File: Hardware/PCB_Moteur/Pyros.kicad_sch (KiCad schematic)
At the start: 33 parts, among them J17 Screw_Terminal_01x04, Q1 SI5442DU-T1-GE3, Q2 SI5442DU-T1-GE3, Q3 MMBT3904, Q4 SI7617DN-T1-GE3, U6 LM393

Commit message: wip : done all footprints
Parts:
- J17: footprint (none) -> pcb_moteur:CONN_OSTVN04A150_OST
- Q1, Q2: footprint SON_8DU-T1-GE3_VIS -> pcb_moteur:SI5442DU_T1_G3
- Q4: footprint POWERPAK_1212-8_VIS -> pcb_moteur:SI7617DN-T1-GE3
- R49, R50: footprint Resistor_SMD:R_0603_1608Metric -> Resistor_SMD:R_0805_2012Metric
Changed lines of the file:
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@@
 			)
 		)
-		(property "Footprint" "Resistor_SMD:R_0603_1608Metric"
+		(property "Footprint" "Resistor_SMD:R_0805_2012Metric"
 			(at 218.948 34.29 90)
 			(effects
@@
 			)
 		)
-		(property "Footprint" "Resistor_SMD:R_0603_1608Metric"
+		(property "Footprint" "Resistor_SMD:R_0805_2012Metric"
 			(at 206.248 57.15 90)
 			(effects
@@
 			)
 		)
-		(property "Footprint" "SON_8DU-T1-GE3_VIS"
+		(property "Footprint" "pcb_moteur:SI5442DU_T1_G3"
 			(at 113.03 133.096 0)
 			(effects
@@
 			)
 		)
-		(property "Footprint" "POWERPAK_1212-8_VIS"
+		(property "Footprint" "pcb_moteur:SI7617DN-T1-GE3"
 			(at 224.79 33.02 0)
 			(effects
@@
 			)
 		)
-		(property "Footprint" "SON_8DU-T1-GE3_VIS"
+		(property "Footprint" "pcb_moteur:SI5442DU_T1_G3"
 			(at 44.45 133.096 0)
 			(effects
@@
 			)
 		)
-		(property "Footprint" ""
+		(property "Footprint" "pcb_moteur:CONN_OSTVN04A150_OST"
 			(at 180.34 100.33 0)
 			(effects
@@
 			)
 		)
-		(property "Datasheet" "~"
+		(property "Datasheet" "https://www.digikey.ca/en/products/detail/on-shore-technology-inc/OSTVN04A150/1588864"
 			(at 180.34 100.33 0)
 			(effects

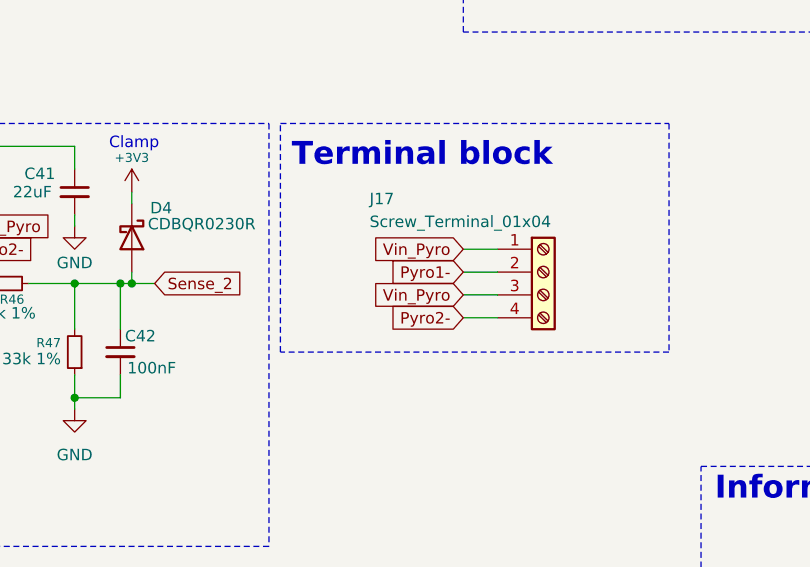
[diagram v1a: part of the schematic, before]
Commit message: wip: layout circuits Pyro
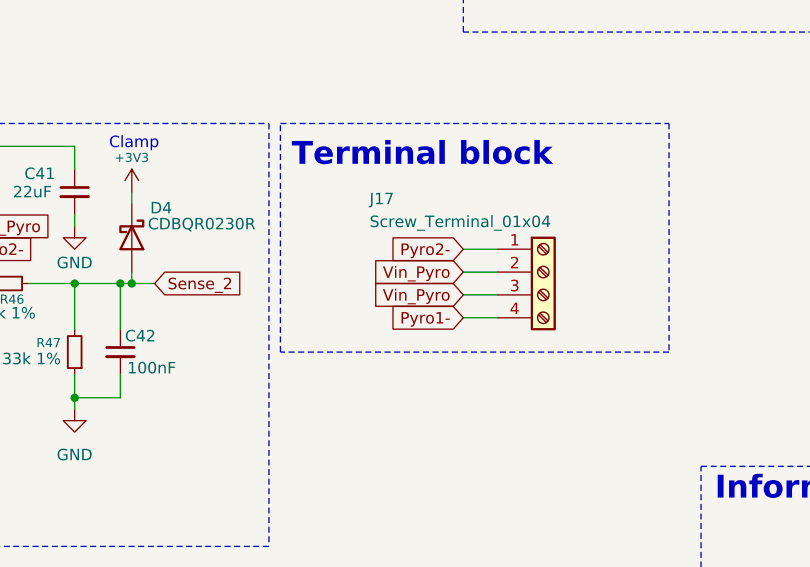
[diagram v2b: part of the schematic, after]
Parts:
- R36, R37, R38, R39, R40, R41, R42, R43, R44, R45, R46, R47, R48, R51, R52: footprint Resistor_SMD:R_0603_1608Metric -> Resistor_SMD:R_0805_2012Metric
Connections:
- net Pyro1-: now also J17.4 (Pin_4); no longer J17.2 (Pin_2)
- net Pyro2-: now also J17.1 (Pin_1); no longer J17.4 (Pin_4)
- net Vin_Pyro: now also J17.2 (Pin_2); no longer J17.1 (Pin_1)
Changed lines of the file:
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@@
 	(wire
 		(pts
+			(xy 171.45 100.33) (xy 175.26 100.33)
+		)
+		(stroke
+			(width 0)
+			(type default)
+		)
+	)
+	(wire
+		(pts
 			(xy 128.27 86.36) (xy 115.57 86.36)
 		)
@@
 	(wire
 		(pts
-			(xy 171.45 97.79) (xy 175.26 97.79)
-		)
-		(stroke
-			(width 0)
-			(type default)
-		)
-	)
-	(wire
-		(pts
 			(xy 134.62 100.33) (xy 134.62 101.6)
 		)
@@
 	(wire
 		(pts
-			(xy 171.45 100.33) (xy 175.26 100.33)
-		)
-		(stroke
-			(width 0)
-			(type default)
-		)
-	)
-	(wire
-		(pts
 			(xy 26.67 43.18) (xy 26.67 48.26)
 		)
@@
 	(wire
 		(pts
+			(xy 171.45 97.79) (xy 175.26 97.79)
+		)
+		(stroke
+			(width 0)
+			(type default)
+		)
+	)
+	(wire
+		(pts
 			(xy 223.52 27.94) (xy 223.52 33.02)
 		)
@@
 	(global_label "Vin_Pyro"
 		(shape input)
-		(at 171.45 97.79 180)
+		(at 171.45 100.33 180)
 		(fields_autoplaced yes)
 		(effects
@@
 		)
 		(property "Intersheetrefs" "${INTERSHEET_REFS}"
-			(at 160.482 97.79 0)
+			(at 160.482 100.33 0)
 			(effects
 				(font
@@
 		)
 	)
-	(global_label "Cmp_2"
+	(global_label "Pyro2-"
 		(shape input)
-		(at 67.31 50.8 0)
+		(at 171.45 97.79 180)
 		(fields_autoplaced yes)
 		(effects
@@
 				(size 1.27 1.27)
 			)
-			(justify left)
+			(justify right)
 		)
 		(property "Intersheetrefs" "${INTERSHEET_REFS}"
-			(at 76.5846 50.8 0)
+			(at 161.5101 97.79 0)
 			(effects
 				(font
 					(size 1.27 1.27)
 				)
-				(justify left)
+				(justify right)
 				(hide yes)
 			)
@@
 	(global_label "Cmp_2"
 		(shape input)
-		(at 92.71 109.22 180)
+		(at 67.31 50.8 0)
 		(fields_autoplaced yes)
 		(effects
@@
 				(size 1.27 1.27)
 			)
-			(justify right)
+			(justify left)
 		)
 		(property "Intersheetrefs" "${INTERSHEET_REFS}"
-			(at 83.4354 109.22 0)
+			(at 76.5846 50.8 0)
 			(effects
 				(font
 					(size 1.27 1.27)
 				)
-				(justify right)
+				(justify left)
 				(hide yes)
 			)
 		)
 	)
-	(global_label "PA_An"
+	(global_label "Cmp_2"
 		(shape input)
-		(at 240.03 62.23 180)
+		(at 92.71 109.22 180)
 		(fields_autoplaced yes)
 		(effects
@@
 		)
 		(property "Intersheetrefs" "${INTERSHEET_REFS}"
-			(at 231.481 62.23 0)
+			(at 83.4354 109.22 0)
 			(effects
 				(font
@@
 		)
 	)
-	(global_label "Vin_Pyro"
+	(global_label "PA_An"
 		(shape input)
-		(at 44.45 86.36 180)
+		(at 240.03 62.23 180)
 		(fields_autoplaced yes)
 		(effects
@@
 		)
 		(property "Intersheetrefs" "${INTERSHEET_REFS}"
-			(at 33.482 86.36 0)
+			(at 231.481 62.23 0)
 			(effects
 				(font
@@
 		)
 	)
-	(global_label "Pyro1-"
+	(global_label "Vin_Pyro"
 		(shape input)
-		(at 171.45 100.33 180)
+		(at 44.45 86.36 180)
 		(fields_autoplaced yes)
 		(effects
@@
 		)
 		(property "Intersheetrefs" "${INTERSHEET_REFS}"
-			(at 161.5101 100.33 0)
+			(at 33.482 86.36 0)
 			(effects
 				(font
@@
 		)
 	)
-	(global_label "Vin_Pyro"
+	(global_label "Pyro1-"
 		(shape input)
-		(at 115.57 95.25 0)
+		(at 171.45 105.41 180)
 		(fields_autoplaced yes)
 		(effects
@@
 				(size 1.27 1.27)
 			)
-			(justify left)
+			(justify right)
 		)
 		(property "Intersheetrefs" "${INTERSHEET_REFS}"
-			(at 126.538 95.25 0)
+			(at 161.5101 105.41 0)
 			(effects
 				(font
 					(size 1.27 1.27)
 				)
-				(justify left)
+				(justify right)
 				(hide yes)
 			)
 		)
 	)
-	(global_label "Pyro2-"
+	(global_label "Vin_Pyro"
 		(shape input)
-		(at 171.45 105.41 180)
+		(at 115.57 95.25 0)
 		(fields_autoplaced yes)
 		(effects
@@
 				(size 1.27 1.27)
 			)
-			(justify right)
+			(justify left)
 		)
 		(property "Intersheetrefs" "${INTERSHEET_REFS}"
-			(at 161.5101 105.41 0)
+			(at 126.538 95.25 0)
 			(effects
 				(font
 					(size 1.27 1.27)
 				)
-				(justify right)
+				(justify left)
 				(hide yes)
 			)
@@
 			)
 		)
-		(property "Footprint" "Resistor_SMD:R_0603_1608Metric"
+		(property "Footprint" "Resistor_SMD:R_0805_2012Metric"
 			(at 31.75 58.42 0)
 			(effects
@@
 			)
 		)
-		(property "Footprint" "Resistor_SMD:R_0603_1608Metric"
+		(property "Footprint" "Resistor_SMD:R_0805_2012Metric"
 			(at 31.75 40.64 0)
 			(effects
@@
 			)
 		)
-		(property "Footprint" "Resistor_SMD:R_0603_1608Metric"
+		(property "Footprint" "Resistor_SMD:R_0805_2012Metric"
 			(at 52.07 101.6 0)
 			(effects
@@
 			)
 		)
-		(property "Footprint" "Resistor_SMD:R_0603_1608Metric"
+		(property "Footprint" "Resistor_SMD:R_0805_2012Metric"
 			(at 248.92 56.388 90)
 			(effects
@@
 			)
 		)
-		(property "Footprint" "Resistor_SMD:R_0603_1608Metric"
+		(property "Footprint" "Resistor_SMD:R_0805_2012Metric"
 			(at 59.69 109.22 0)
 			(effects
@@
 			)
 		)
-		(property "Footprint" "Resistor_SMD:R_0603_1608Metric"
+		(property "Footprint" "Resistor_SMD:R_0805_2012Metric"
 			(at 26.67 40.64 0)
 			(effects
@@
 			)
 		)
-		(property "Footprint" "Resistor_SMD:R_0603_1608Metric"
+		(property "Footprint" "Resistor_SMD:R_0805_2012Metric"
 			(at 101.6 115.57 0)
 			(effects
@@
 			)
 		)
-		(property "Footprint" "Resistor_SMD:R_0603_1608Metric"
+		(property "Footprint" "Resistor_SMD:R_0805_2012Metric"
 			(at 26.67 58.42 0)
 			(effects
@@
 			)
 		)
-		(property "Footprint" "Resistor_SMD:R_0603_1608Metric"
+		(property "Footprint" "Resistor_SMD:R_0805_2012Metric"
 			(at 120.65 101.6 0)
 			(effects
@@
 			)
 		)
-		(property "Footprint" "Resistor_SMD:R_0603_1608Metric"
+		(property "Footprint" "Resistor_SMD:R_0805_2012Metric"
 			(at 261.62 56.388 90)
 			(effects
@@
 			)
 		)
-		(property "Footprint" "Resistor_SMD:R_0603_1608Metric"
+		(property "Footprint" "Resistor_SMD:R_0805_2012Metric"
 			(at 27.94 119.38 0)
 			(effects
@@
 			)
 		)
-		(property "Footprint" "Resistor_SMD:R_0603_1608Metric"
+		(property "Footprint" "Resistor_SMD:R_0805_2012Metric"
 			(at 128.27 109.22 0)
 			(effects
@@
 			)
 		)
-		(property "Footprint" "Resistor_SMD:R_0603_1608Metric"
+		(property "Footprint" "Resistor_SMD:R_0805_2012Metric"
 			(at 96.52 119.38 0)
 			(effects
@@
 			)
 		)
-		(property "Footprint" "Resistor_SMD:R_0603_1608Metric"
+		(property "Footprint" "Resistor_SMD:R_0805_2012Metric"
 			(at 198.12 47.752 90)
 			(effects
@@
 			)
 		)
-		(property "Footprint" "Resistor_SMD:R_0603_1608Metric"
+		(property "Footprint" "Resistor_SMD:R_0805_2012Metric"
 			(at 33.02 115.57 0)
 			(effects
